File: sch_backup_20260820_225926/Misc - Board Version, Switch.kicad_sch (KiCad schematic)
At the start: 11 parts, among them SW1 DSIC02LSGET

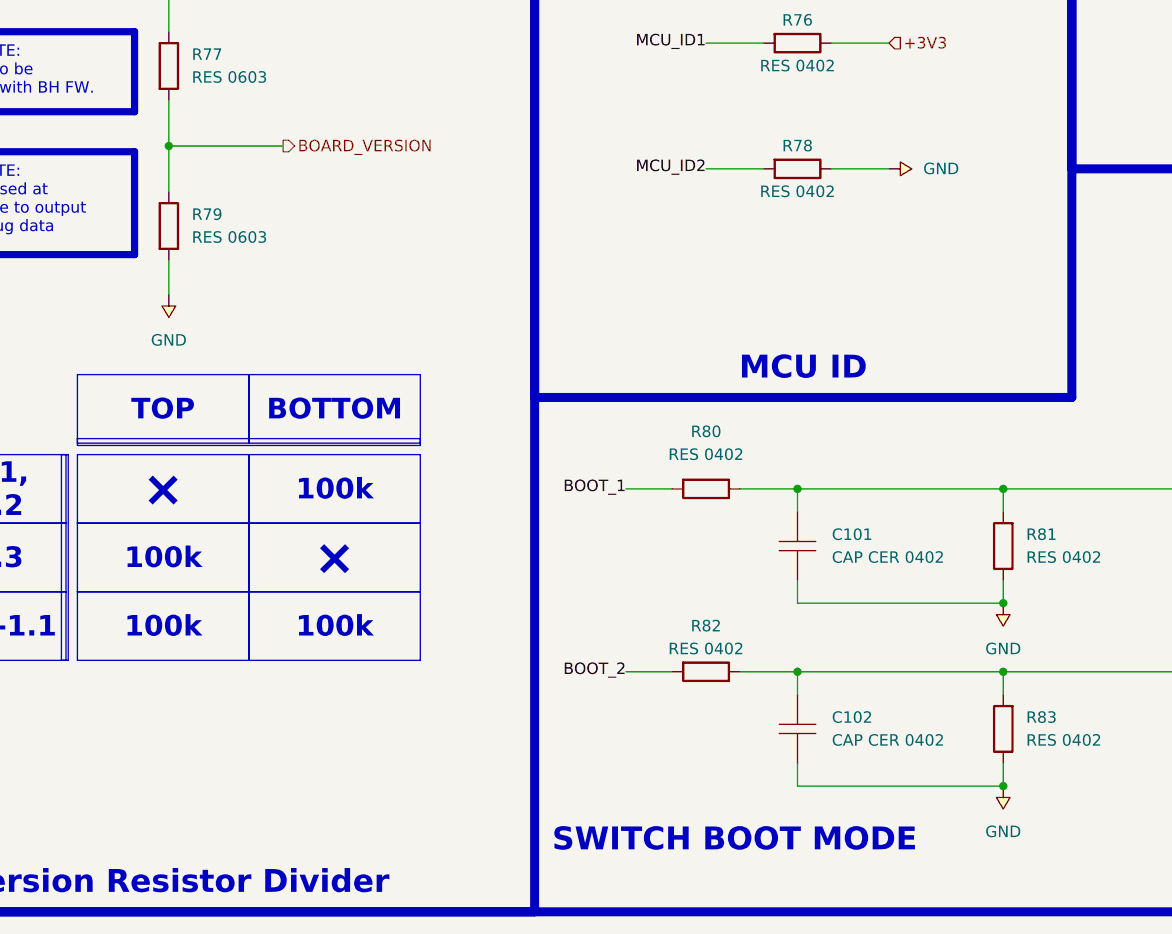
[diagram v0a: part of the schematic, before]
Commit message: Update Schematic
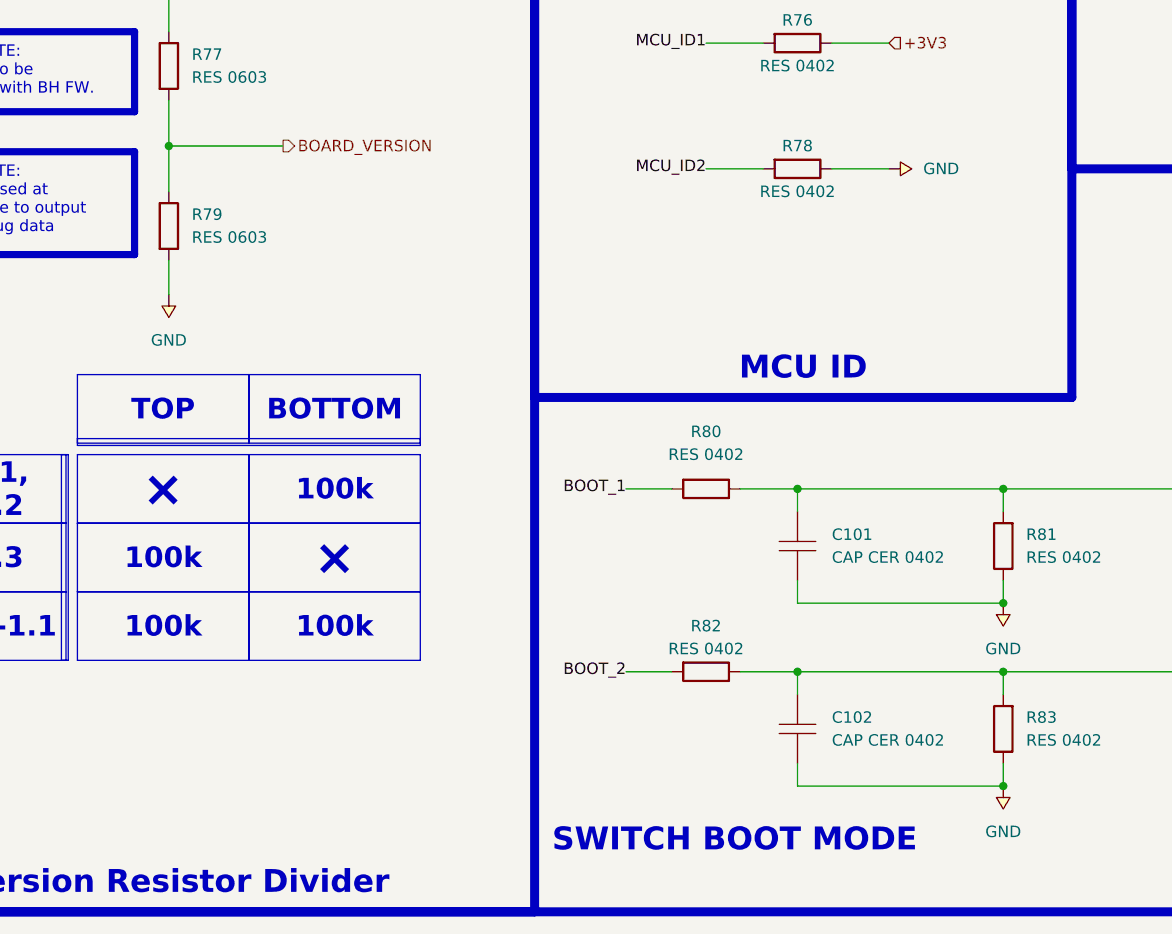
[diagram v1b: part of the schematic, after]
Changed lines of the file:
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@@
 	)
 	(junction
-		(at 182.88 118.11)
+		(at 233.68 105.41)
 		(diameter 0)
 		(color 0 0 0 0)
 	)
 	(junction
-		(at 182.88 138.43)
+		(at 182.88 125.73)
 		(diameter 0)
 		(color 0 0 0 0)
 	)
 	(junction
-		(at 233.68 105.41)
+		(at 90.17 67.31)
 		(diameter 0)
 		(color 0 0 0 0)
 	)
 	(junction
-		(at 182.88 125.73)
+		(at 182.88 118.11)
 		(diameter 0)
 		(color 0 0 0 0)
 	)
 	(junction
-		(at 90.17 67.31)
+		(at 182.88 138.43)
 		(diameter 0)
 		(color 0 0 0 0)
@@
 	(symbol
 		(lib_id "Power_symbols:GND")
-		(at 92.71 83.82 0)
+		(at 90.17 82.55 180)
 		(unit 1)
 		(exclude_from_sim no)
@@
 		(dnp no)
 		(fields_autoplaced yes)
-		(property "Reference" "#PWR0137"
-			(at 92.456 75.184 0)
+		(property "Reference" "#PWR133"
+			(at 90.17 82.55 0)
 			(do_not_autoplace yes)
 			(effects
@@
 		)
 		(property "Footprint" ""
-			(at 92.71 83.82 0)
+			(at 90.17 82.55 0)
 			(effects
 				(font
@@
 		)
 		(property "Datasheet" ""
-			(at 92.71 83.82 0)
+			(at 90.17 82.55 0)
 			(effects
 				(font
@@
 		)
 		(property "Description" "Power Symbol - Global Ground"
-			(at 92.71 90.678 0)
+			(at 90.17 82.55 0)
 			(effects
 				(font
@@
 			(project "Master_Hand_Kicad"
 				(path "/f9e05184-c88b-4a88-ae9c-ab2bdb32be7c/c5103ceb-5325-4a84-a025-9638a412984e/0bb1cb44-88fa-40dc-bea3-1adee4cb244a"
-					(reference "#PWR0137")
+					(reference "#PWR133")
 					(unit 1)
 				)
@@
 	(symbol
 		(lib_id "Power_symbols:GND")
-		(at 170.18 67.31 90)
+		(at 168.91 69.85 270)
 		(unit 1)
 		(exclude_from_sim no)
@@
 		(dnp no)
 		(fields_autoplaced yes)
-		(property "Reference" "#PWR0136"
-			(at 161.544 67.564 0)
+		(property "Reference" "#PWR132"
+			(at 168.91 69.85 0)
 			(do_not_autoplace yes)
 			(effects
@@
 					(size 1.27 1.27)
 				)
-				(justify right)
+				(justify left)
 			)
 		)
 		(property "Footprint" ""
-			(at 170.18 67.31 0)
+			(at 168.91 69.85 0)
 			(effects
 				(font
@@
 		)
 		(property "Datasheet" ""
-			(at 170.18 67.31 0)
+			(at 168.91 69.85 0)
 			(effects
 				(font
@@
 		)
 		(property "Description" "Power Symbol - Global Ground"
-			(at 177.038 67.31 0)
+			(at 168.91 69.85 0)
 			(effects
 				(font
@@
 			(project "Master_Hand_Kicad"
 				(path "/f9e05184-c88b-4a88-ae9c-ab2bdb32be7c/c5103ceb-5325-4a84-a025-9638a412984e/0bb1cb44-88fa-40dc-bea3-1adee4cb244a"
-					(reference "#PWR0136")
+					(reference "#PWR132")
 					(unit 1)
 				)
@@
 	(symbol
 		(lib_id "Power_symbols:GND")
-		(at 185.42 138.43 0)
+		(at 182.88 137.16 180)
 		(unit 1)
 		(exclude_from_sim no)
@@
 		(dnp no)
 		(fields_autoplaced yes)
-		(property "Reference" "#PWR0139"
-			(at 185.166 129.794 0)
+		(property "Reference" "#PWR135"
+			(at 182.88 137.16 0)
 			(do_not_autoplace yes)
 			(effects
@@
 		)
 		(property "Footprint" ""
-			(at 185.42 138.43 0)
+			(at 182.88 137.16 0)
 			(effects
 				(font
@@
 		)
 		(property "Datasheet" ""
-			(at 185.42 138.43 0)
+			(at 182.88 137.16 0)
 			(effects
 				(font
@@
 		)
 		(property "Description" "Power Symbol - Global Ground"
-			(at 185.42 145.288 0)
+			(at 182.88 137.16 0)
 			(effects
 				(font
@@
 			(project "Master_Hand_Kicad"
 				(path "/f9e05184-c88b-4a88-ae9c-ab2bdb32be7c/c5103ceb-5325-4a84-a025-9638a412984e/0bb1cb44-88fa-40dc-bea3-1adee4cb244a"
-					(reference "#PWR0139")
+					(reference "#PWR135")
 					(unit 1)
 				)
@@
 	(symbol
 		(lib_id "Power_symbols:GND")
-		(at 185.42 118.11 0)
+		(at 182.88 116.84 180)
 		(unit 1)
 		(exclude_from_sim no)
@@
 		(dnp no)
 		(fields_autoplaced yes)
-		(property "Reference" "#PWR0138"
-			(at 185.166 109.474 0)
+		(property "Reference" "#PWR134"
+			(at 182.88 116.84 0)
 			(do_not_autoplace yes)
 			(effects
@@
 		)
 		(property "Footprint" ""
-			(at 185.42 118.11 0)
+			(at 182.88 116.84 0)
 			(effects
 				(font
@@
 		)
 		(property "Datasheet" ""
-			(at 185.42 118.11 0)
+			(at 182.88 116.84 0)
 			(effects
 				(font
@@
 		)
 		(property "Description" "Power Symbol - Global Ground"
-			(at 185.42 124.968 0)
+			(at 182.88 116.84 0)
 			(effects
 				(font
@@
 			(project "Master_Hand_Kicad"
 				(path "/f9e05184-c88b-4a88-ae9c-ab2bdb32be7c/c5103ceb-5325-4a84-a025-9638a412984e/0bb1cb44-88fa-40dc-bea3-1adee4cb244a"
-					(reference "#PWR0138")
+					(reference "#PWR134")
 					(unit 1)
 				)
